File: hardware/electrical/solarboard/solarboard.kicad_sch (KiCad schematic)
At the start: 10 parts, among them J1 Conn_01x02_Pin

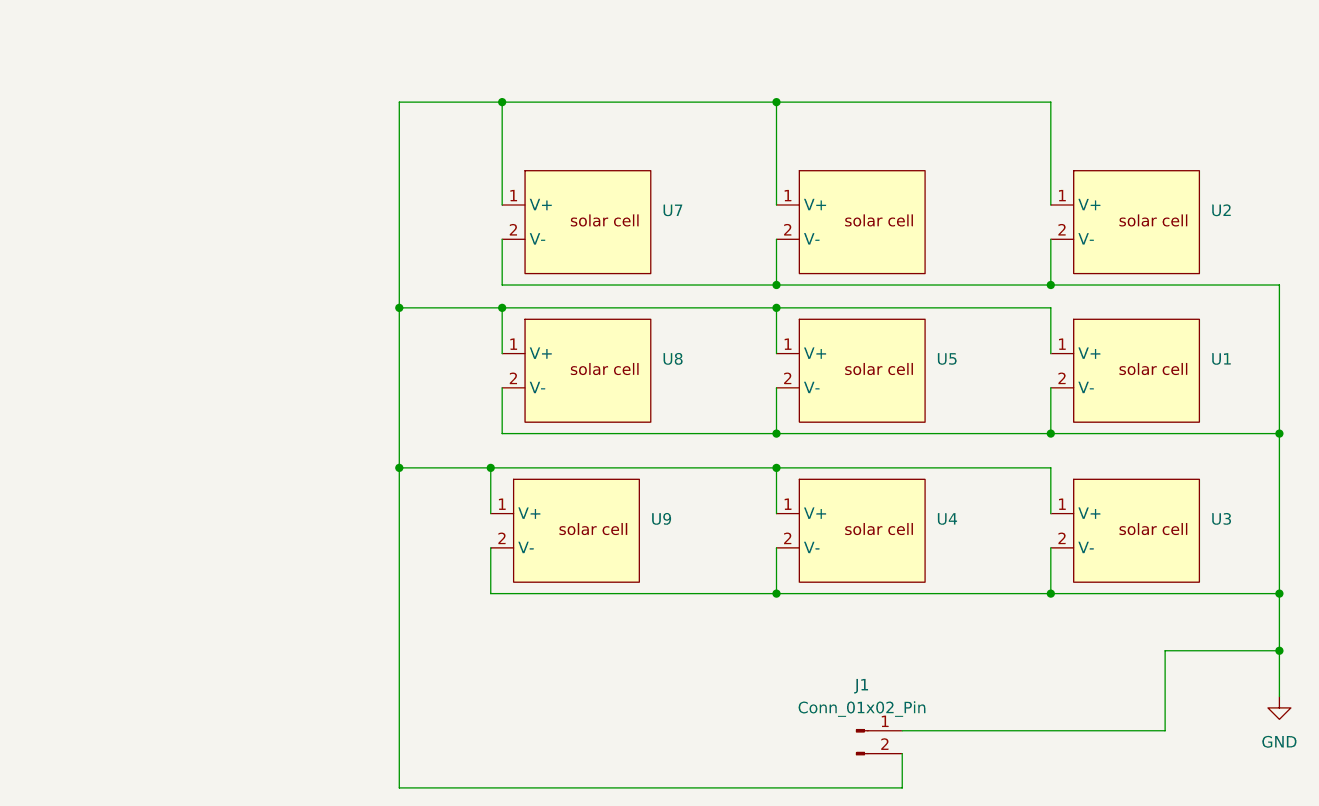
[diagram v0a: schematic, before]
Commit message: update designs and firmware
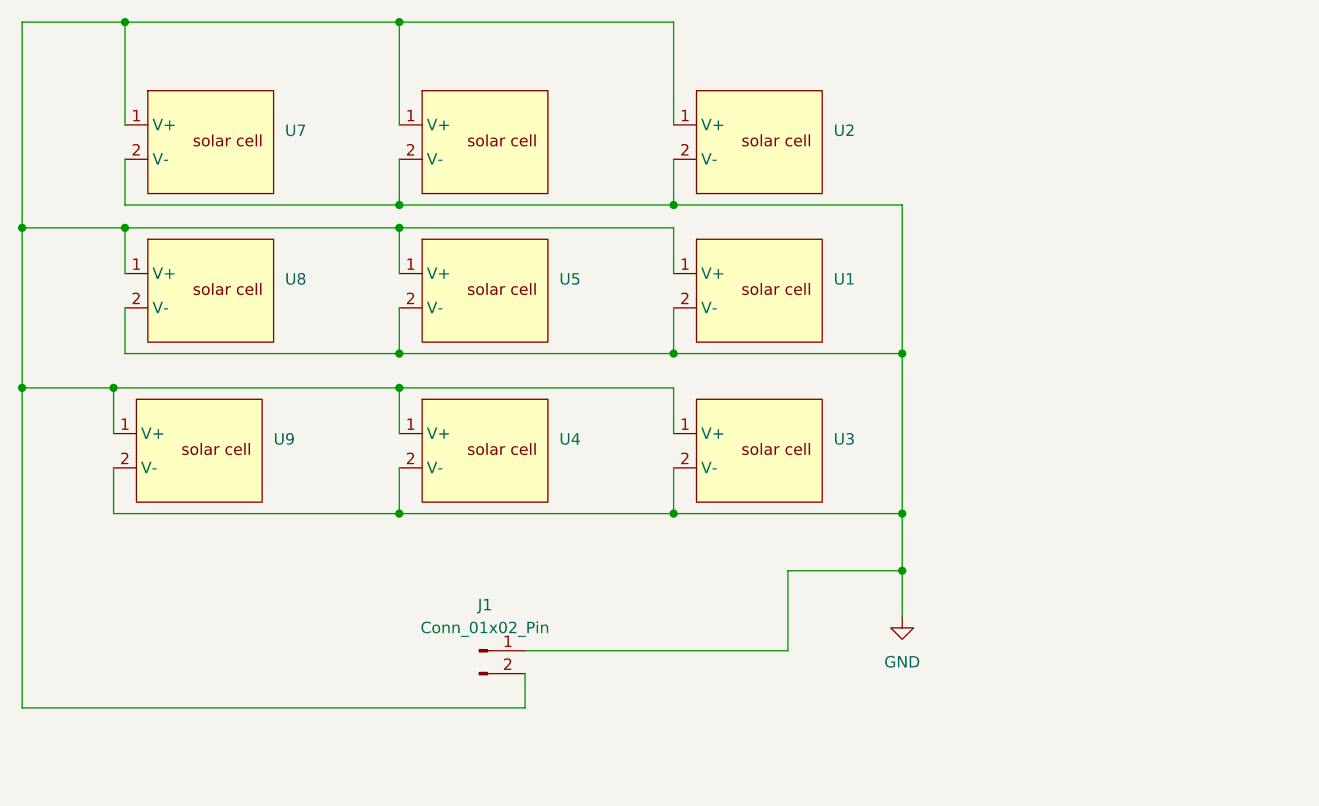
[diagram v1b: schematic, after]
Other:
- moved on the sheet: J1, U1, U2, U3, U4, U5, U7, U8, U9
